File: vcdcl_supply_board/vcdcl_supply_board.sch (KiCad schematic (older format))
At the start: 19 parts, among them J1 Conn_01x02_Male, Q1 IRFR9024, Q2 Q_NPN_ECB, Q3 Q_NPN_BCE, SW1 SW_DIP_x01

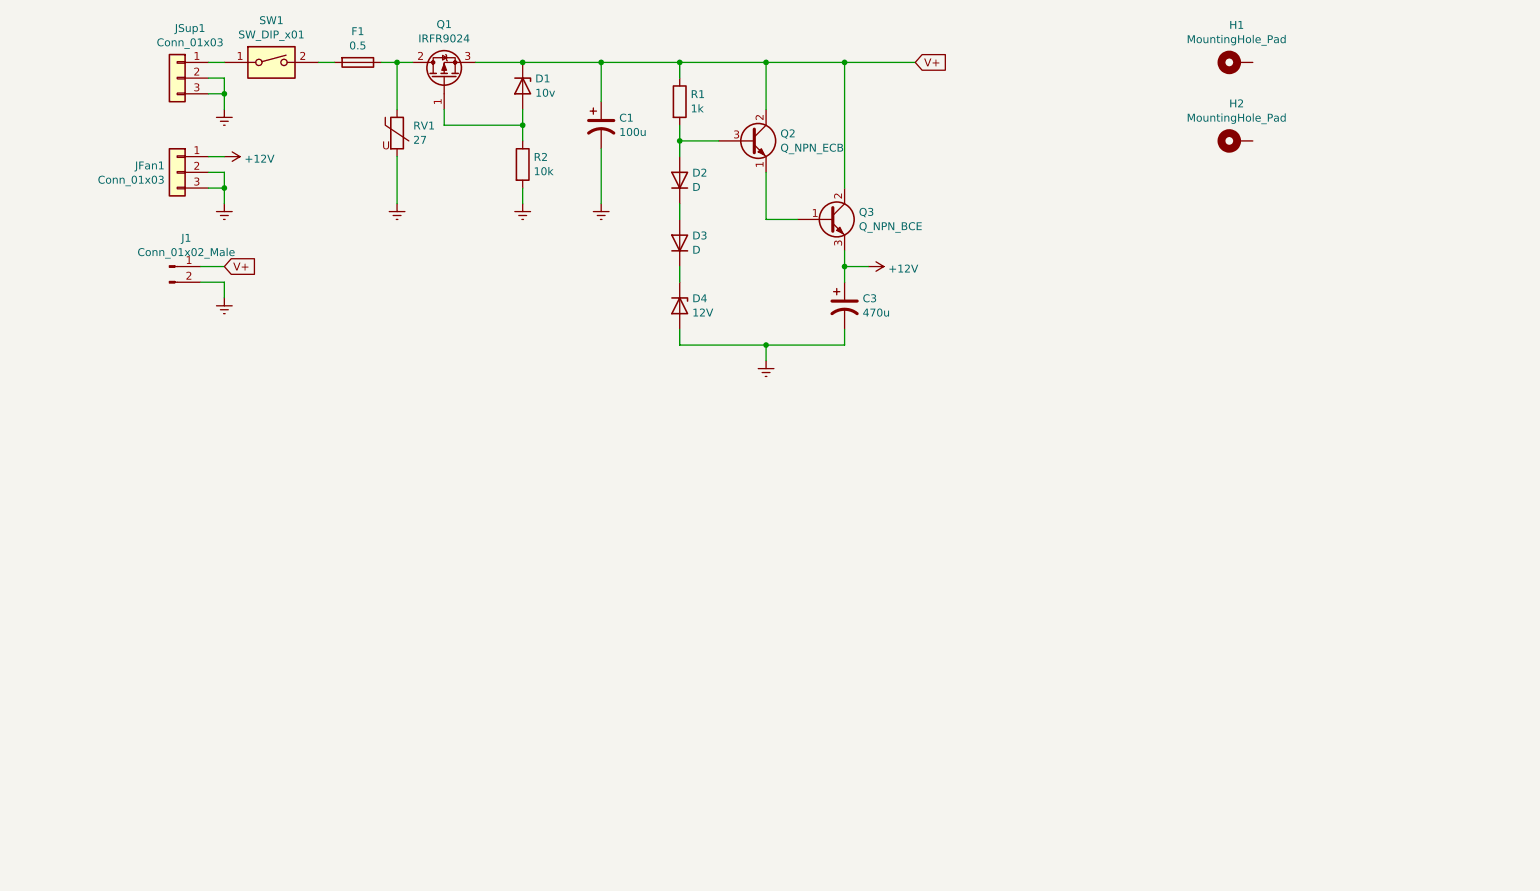
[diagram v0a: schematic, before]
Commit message: Supply board fixes
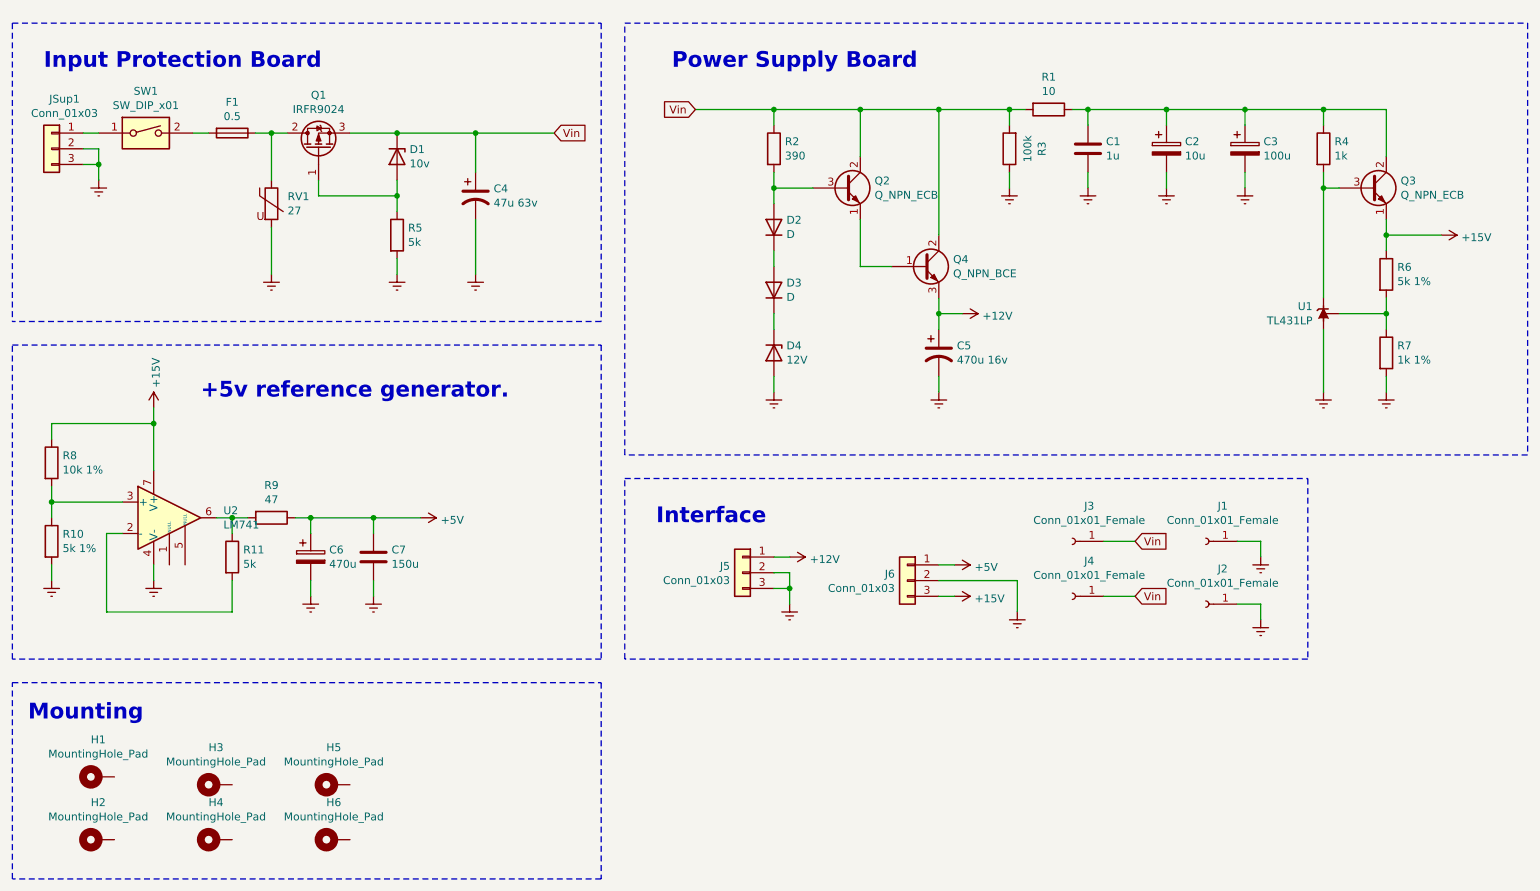
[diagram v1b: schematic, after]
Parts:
- removed J1: Conn_01x02_Male, _сustom:LUT_PinHeader_1x02_P2.54mm_Vertical, symbol Connector:Conn_01x02_Male
- added C1: 1u, _сustom:LUT_C_Rect_L7.0mm_W4.5mm_P5.00mm, symbol Device:C
- added C2: 10u, _сustom:LUT_CP_Radial_D4.0mm_P2.00mm, symbol Device:CP
- added C3: 100u, _сustom:LUT_CP_Radial_D6.3mm_P2.50mm, symbol Device:CP
- added C6: 470u, _сustom:LUT_CP_Radial_D6.3mm_P2.50mm, symbol Device:CP
- added C7: 150u, _сustom:LUT_C_Rect_L10.3mm_W5.0mm_P7.50mm, symbol Device:C
- added H3, H4, H5, H6: MountingHole_Pad, MountingHole:MountingHole_3.2mm_M3_ISO7380_Pad, symbol Mechanical:MountingHole_Pad
- added J1, J2, J3, J4: Conn_01x01_Female, _сustom:LUT_PinHeader_1x01_P2.54mm_Vertical, symbol Connector:Conn_01x01_Female
- added J5: Conn_01x03, _сustom:LUT_FanPinHeader_1x03_P2.54mm_Vertical, symbol Connector_Generic:Conn_01x03
- added Q3: Q_NPN_ECB, _сustom:LUT_TO-92, symbol Device:Q_NPN_ECB
- added R1: 10, _сustom:LUT_R_L6.3mm_D2.5mm_P7.62mm_Horizontal, symbol Device:R
- added R10, R6: 5k 1%, _сustom:LUT_R_L6.3mm_D2.5mm_P7.62mm_Horizontal, symbol Device:R
- added R11: 5k, _сustom:LUT_R_L6.3mm_D2.5mm_P7.62mm_Horizontal, symbol Device:R
- added R3: 100k, _сustom:LUT_R_L6.3mm_D2.5mm_P7.62mm_Horizontal, symbol Device:R
- added R4: 1k, _сustom:LUT_R_L6.3mm_D2.5mm_P7.62mm_Horizontal, symbol Device:R
- added R7: 1k 1%, _сustom:LUT_R_L6.3mm_D2.5mm_P7.62mm_Horizontal, symbol Device:R
- added R8: 10k 1%, _сustom:LUT_R_L6.3mm_D2.5mm_P7.62mm_Horizontal, symbol Device:R
- added R9: 47, _сustom:LUT_R_L6.3mm_D2.5mm_P7.62mm_Horizontal, symbol Device:R
- added U1: TL431LP, _сustom:LUT_TO-92, symbol Reference_Voltage:TL431LP
- added U2: LM741, _сustom:LUT_DIP-8, symbol Amplifier_Operational:LM741
- C4: renamed from C1; value 100u -> 47u 63v; footprint _сustom:LUT_CP_Radial_D6.3mm_P2.50mm -> _сustom:LUT_CP_Radial_D8.0mm_P2.50mm
- C5: renamed from C3; value 470u -> 470u 16v
- D1: footprint _сustom:LUT_D_P7.62mm_Horizontal -> _сustom:LUT_D_P10.16mm_Horizontal
- R2: renamed from R1; value 1k -> 390
- R5: renamed from R2; value 10k -> 5k
- renumbered JFan1 to J6, Q3 to Q4
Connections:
- net +12V: now also J5.1 (Pin_1); no longer J6.1 (Pin_1)
- net Earth: now also C1.2, C2.2, C3.2, C6.2, C7.2, J1.1 (Pin_1), J2.1 (Pin_1), J5.2 (Pin_2), J5.3 (Pin_3), R10.2, R3.1, R7.2, U1.2 (A), U2.4 (V-); no longer J6.3 (Pin_3)
- net V+ renamed Vin
- net Vin: now also J3.1 (Pin_1), J4.1 (Pin_1), R1.2, R3.2
- new net: C1.1, C2.1, C3.1, Q3.2 (C), R1.1, R4.1
- new net: R6.2, R7.1, U1.1 (REF)
- new net: Q3.3 (B), R4.2, U1.3 (K)
- new net: R11.2, U2.2 (-)
- new net: R10.1, R8.2, U2.3 (+)
- new net: R11.1, R9.2, U2.6
- new net +15V: J6.3 (Pin_3), Q3.1 (E), R6.1, R8.1, U2.7 (V+)
- new net +5V: C6.1, C7.1, J6.1 (Pin_1), R9.1
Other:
- note added: "+5v reference generator."
- note added: "Input Protection Board"
- note added: "Interface"
- note added: "Mounting"
- note added: "Power Supply Board"
- moved on the sheet: C4, C5, D1, D2, D3, D4, F1, H1, H2, J6, JSup1, Q1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
